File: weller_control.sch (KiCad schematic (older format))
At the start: 20 parts, among them J2 AudioJack3_Ground_SwitchR, Q1 AON7403, U2 LTC4440IS6, U3 MCP603-xCH

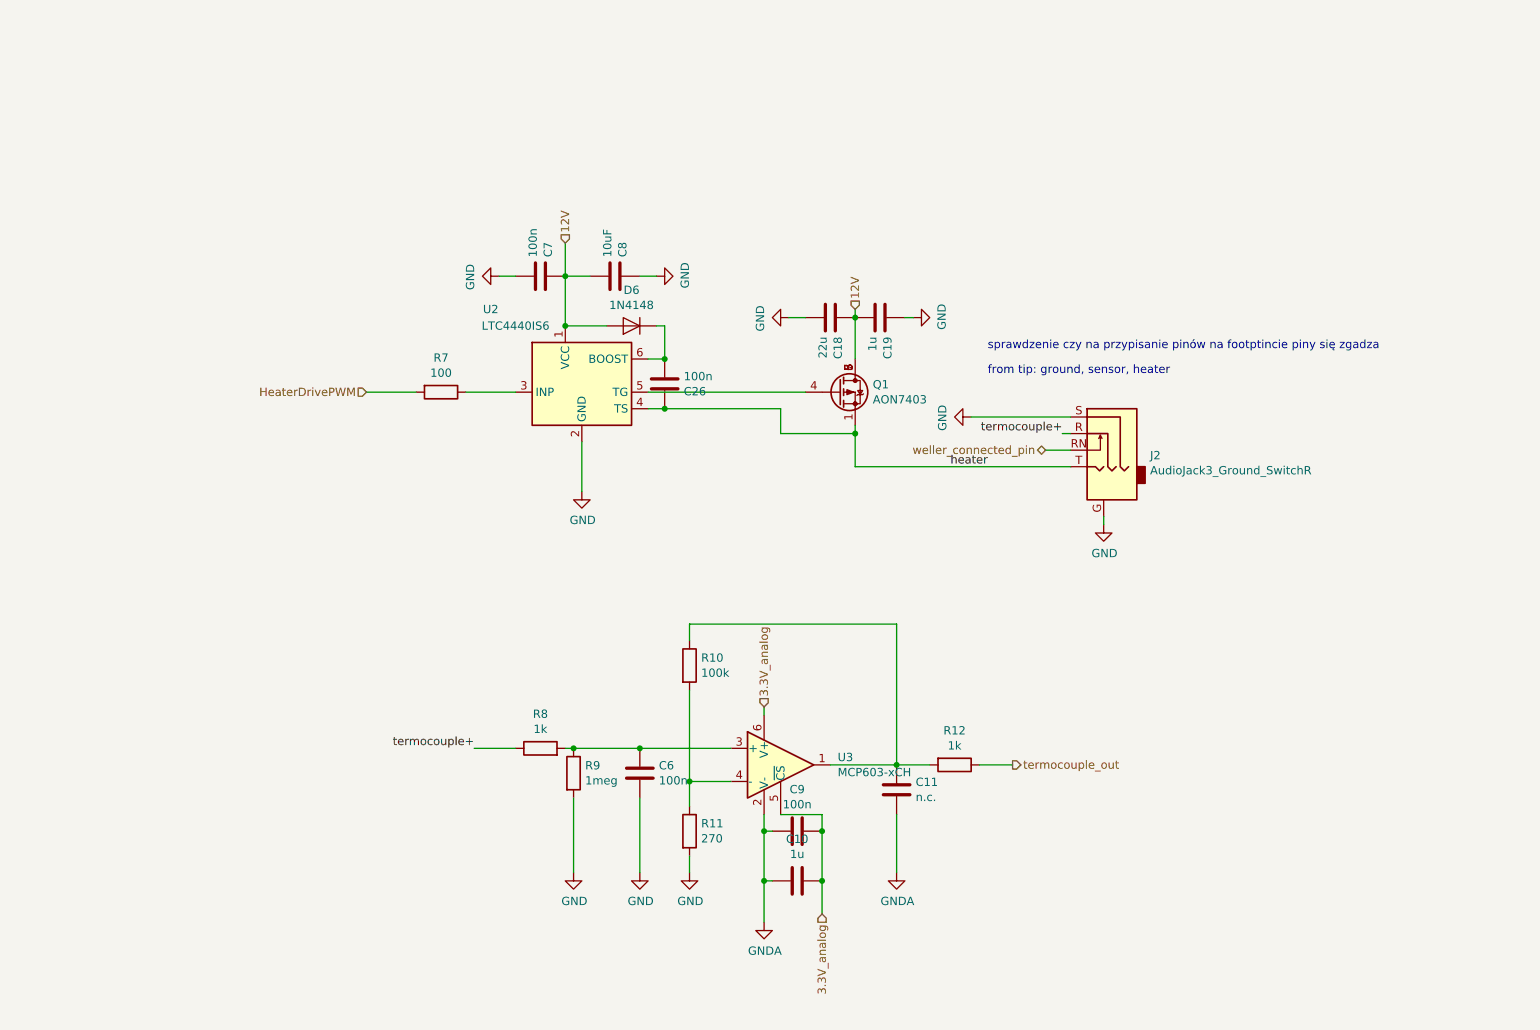
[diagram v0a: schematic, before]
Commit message: update front endu do termopary i przełącznika zasilającego
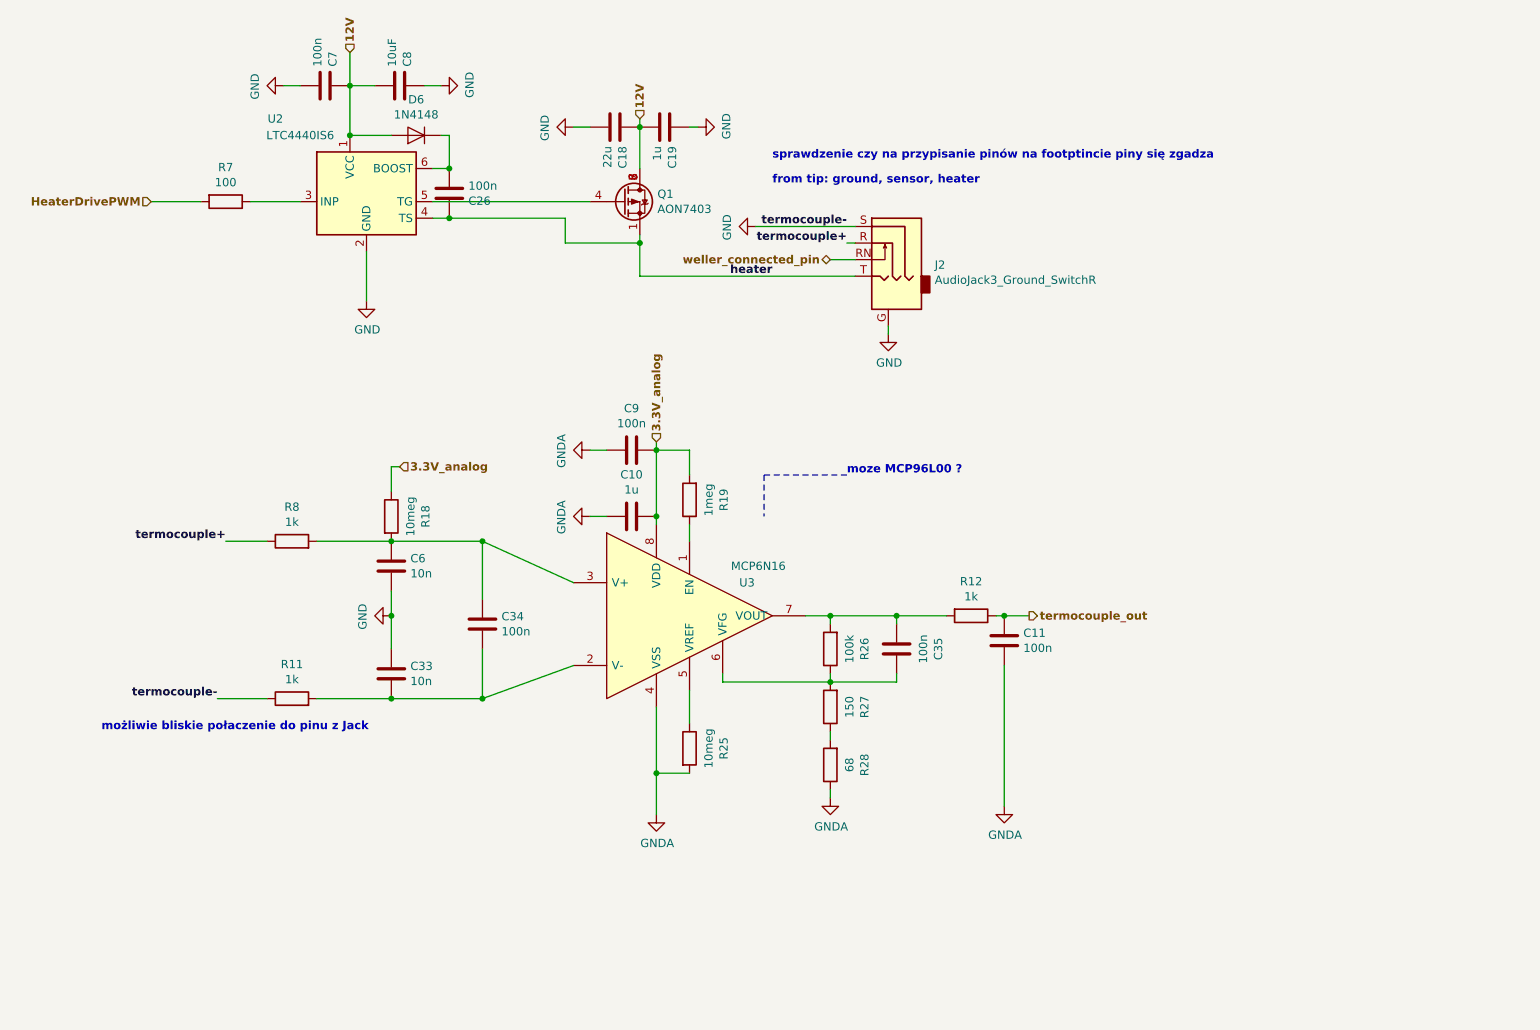
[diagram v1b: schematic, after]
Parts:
- removed R10: 100k, Resistor_SMD:R_0603_1608Metric, symbol Device:R
- removed R9: 1meg, Resistor_SMD:R_0603_1608Metric, symbol Device:R
- removed U3: MCP603-xCH, TO_SOT_Packages_SMD:SOT-23-6, symbol Amplifier_Operational:MCP603-xCH
- added C33: 10n, Capacitor_SMD:C_0603_1608Metric_Pad1.05x0.95mm_HandSolder, symbol Device:C
- added C34, C35: 100n, Capacitor_SMD:C_0603_1608Metric_Pad1.05x0.95mm_HandSolder, symbol Device:C
- added R18, R25: 10meg, Resistor_SMD:R_0603_1608Metric, symbol Device:R
- added R19: 1meg, Resistor_SMD:R_0603_1608Metric, symbol Device:R
- added R26: 100k, Resistor_SMD:R_0603_1608Metric, symbol Device:R
- added R27: 150, Resistor_SMD:R_0603_1608Metric, symbol Device:R
- added R28: 68, Resistor_SMD:R_0603_1608Metric, symbol Device:R
- added U3: MCP6N16, Package_SO:MSOP-8_3x3mm_P0.65mm, symbol russian-nixies:MCP6N16
- C11: value n.c. -> 100n
- C6: value 100n -> 10n
- R11: value 270 -> 1k
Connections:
- net 3.3V_analog: now also R18.1, R19.2, U3.8 (VDD)
- net GND: now also R11.1, C33.1; no longer R11.2
- net GNDA: now also R25.2, R28.1, U3.4 (VSS)
- net termocouple_out: now also C11.1
- net at R12.2: now also C35.1, R26.2, U3.7 (VOUT); no longer C11.1
- net at C6.1, R8.2: now also C34.1, R18.2, U3.3 (V+)
- new net: R19.1, U3.1 (EN)
- new net: C33.2, C34.2, R11.2, U3.2 (V-)
- new net: R25.1, U3.5 (VREF)
- new net: C35.2, R26.1, R27.2, U3.6 (VFG)
- new net: R27.1, R28.2
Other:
- note added: "moze MCP96L00 ?"
- note added: "możliwie bliskie połaczenie do pinu z Jack\n"
- moved on the sheet: C10, C11, C18, C19, C26, C6, C7, C8, C9, D6, J2, Q1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
